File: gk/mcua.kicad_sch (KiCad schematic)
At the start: 16 parts, among them SW1 SW_Push, SW2 SW_Push, U4 STM32H747BITx, Y1 16MHz

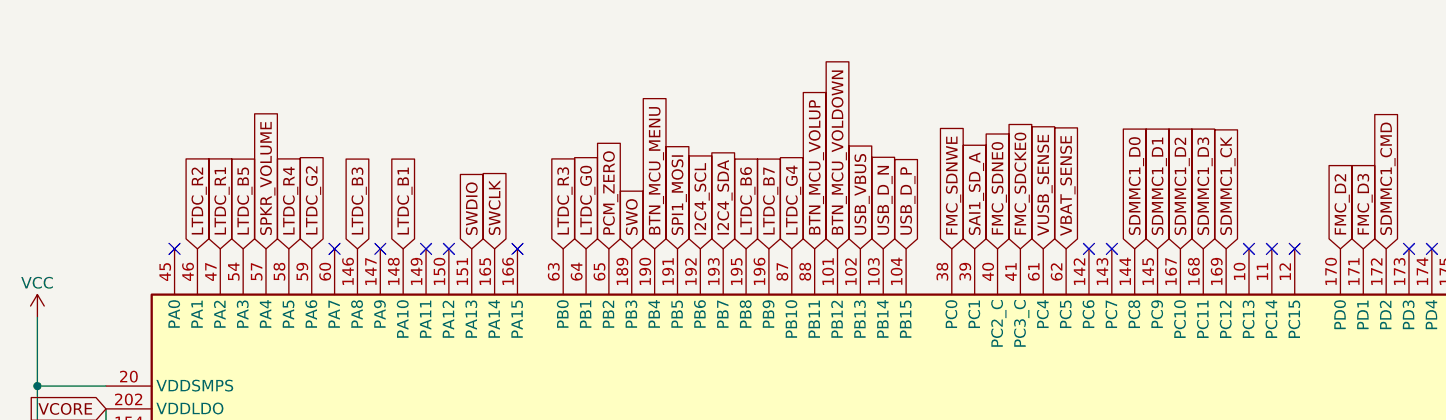
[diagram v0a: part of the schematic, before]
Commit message: Update pcb
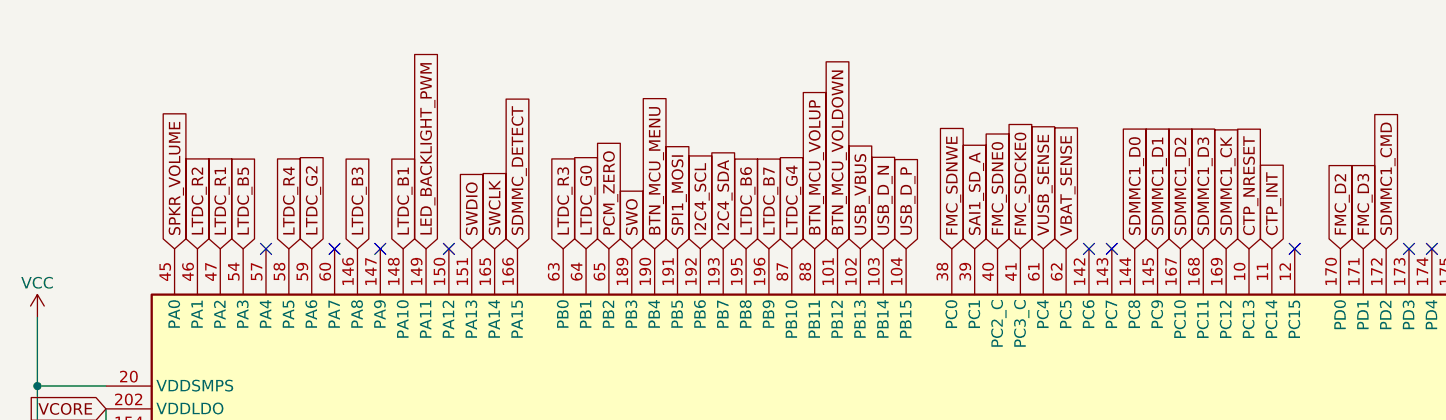
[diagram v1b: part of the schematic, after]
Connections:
- net SPKR_VOLUME: now also U4.45 (PA0); no longer U4.57 (PA4)
- net CTP_NRESET: now reaches U4.10 (PC13)
- net CTP_INT: now reaches U4.11 (PC14)
- net LED_BACKLIGHT_PWM: now reaches U4.149 (PA11)
- net SDMMC_DETECT: now reaches U4.166 (PA15)
- no-connect marks 26 -> 22
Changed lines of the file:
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@@
   (no_connect (at 68.58 146.05))
   (no_connect (at 71.12 146.05))
-  (no_connect (at 73.66 49.53))
-  (no_connect (at 35.56 49.53))
   (no_connect (at 99.06 146.05))
   (no_connect (at 139.7 49.53))
+  (no_connect (at 45.72 49.53))
   (no_connect (at 175.26 49.53))
   (no_connect (at 172.72 49.53))
@@
   (no_connect (at 165.1 146.05))
   (no_connect (at 63.5 146.05))
-  (no_connect (at 154.94 49.53))
   (no_connect (at 66.04 146.05))
-  (no_connect (at 63.5 49.53))
-  (no_connect (at 157.48 49.53))
   (no_connect (at 50.8 146.05))
   (no_connect (at 160.02 49.53))
@@
     )
   )
+  (global_label "CTP_INT" (shape input) (at 157.48 49.53 90) (fields_autoplaced)
+    (effects (font (size 1.27 1.27)) (justify left))
+    (property "Intersheetrefs" "${INTERSHEET_REFS}" (at 157.48 39.2461 90)
+      (effects (font (size 1.27 1.27)) (justify left) hide)
+    )
+  )
   (global_label "WIFI_CHIP_EN" (shape input) (at 195.58 49.53 90) (fields_autoplaced)
     (effects (font (size 1.27 1.27)) (justify left))
@@
     )
   )
+  (global_label "LED_BACKLIGHT_PWM" (shape input) (at 63.5 49.53 90) (fields_autoplaced)
+    (effects (font (size 1.27 1.27)) (justify left))
+    (property "Intersheetrefs" "${INTERSHEET_REFS}" (at 63.5 26.9695 90)
+      (effects (font (size 1.27 1.27)) (justify left) hide)
+    )
+  )
   (global_label "PCM_FMT" (shape input) (at 88.9 146.05 270) (fields_autoplaced)
     (effects (font (size 1.27 1.27)) (justify right))
@@
     )
   )
-  (global_label "SPKR_VOLUME" (shape input) (at 45.72 49.53 90) (fields_autoplaced)
-    (effects (font (size 1.27 1.27)) (justify left))
-    (property "Intersheetrefs" "${INTERSHEET_REFS}" (at 45.72 33.259 90)
-      (effects (font (size 1.27 1.27)) (justify left) hide)
-    )
-  )
   (global_label "FMC_BA1" (shape input) (at 170.18 146.05 270) (fields_autoplaced)
     (effects (font (size 1.27 1.27)) (justify right))
@@
     )
   )
+  (global_label "CTP_NRESET" (shape input) (at 154.94 49.53 90) (fields_autoplaced)
+    (effects (font (size 1.27 1.27)) (justify left))
+    (property "Intersheetrefs" "${INTERSHEET_REFS}" (at 154.94 35.0734 90)
+      (effects (font (size 1.27 1.27)) (justify left) hide)
+    )
+  )
   (global_label "LTDC_HYSNC" (shape input) (at 104.14 146.05 270) (fields_autoplaced)
     (effects (font (size 1.27 1.27)) (justify right))
@@
       (effects (font (size 1.27 1.27)) (justify left) hide)
     )
+  )
+  (global_label "SPKR_VOLUME" (shape input) (at 35.56 49.53 90) (fields_autoplaced)
+    (effects (font (size 1.27 1.27)) (justify left))
+    (property "Intersheetrefs" "${INTERSHEET_REFS}" (at 35.56 33.259 90)
+      (effects (font (size 1.27 1.27)) (justify left) hide)
+    )
+  )
+  (global_label "SDMMC_DETECT" (shape input) (at 73.66 49.53 90) (fields_autoplaced)
+    (effects (font (size 1.27 1.27)) (justify left))
+    (property "Intersheetrefs" "${INTERSHEET_REFS}" (at 73.66 32.2311 90)
+      (effects (font (size 1.27 1.27)) (justify left) hide)
+    )

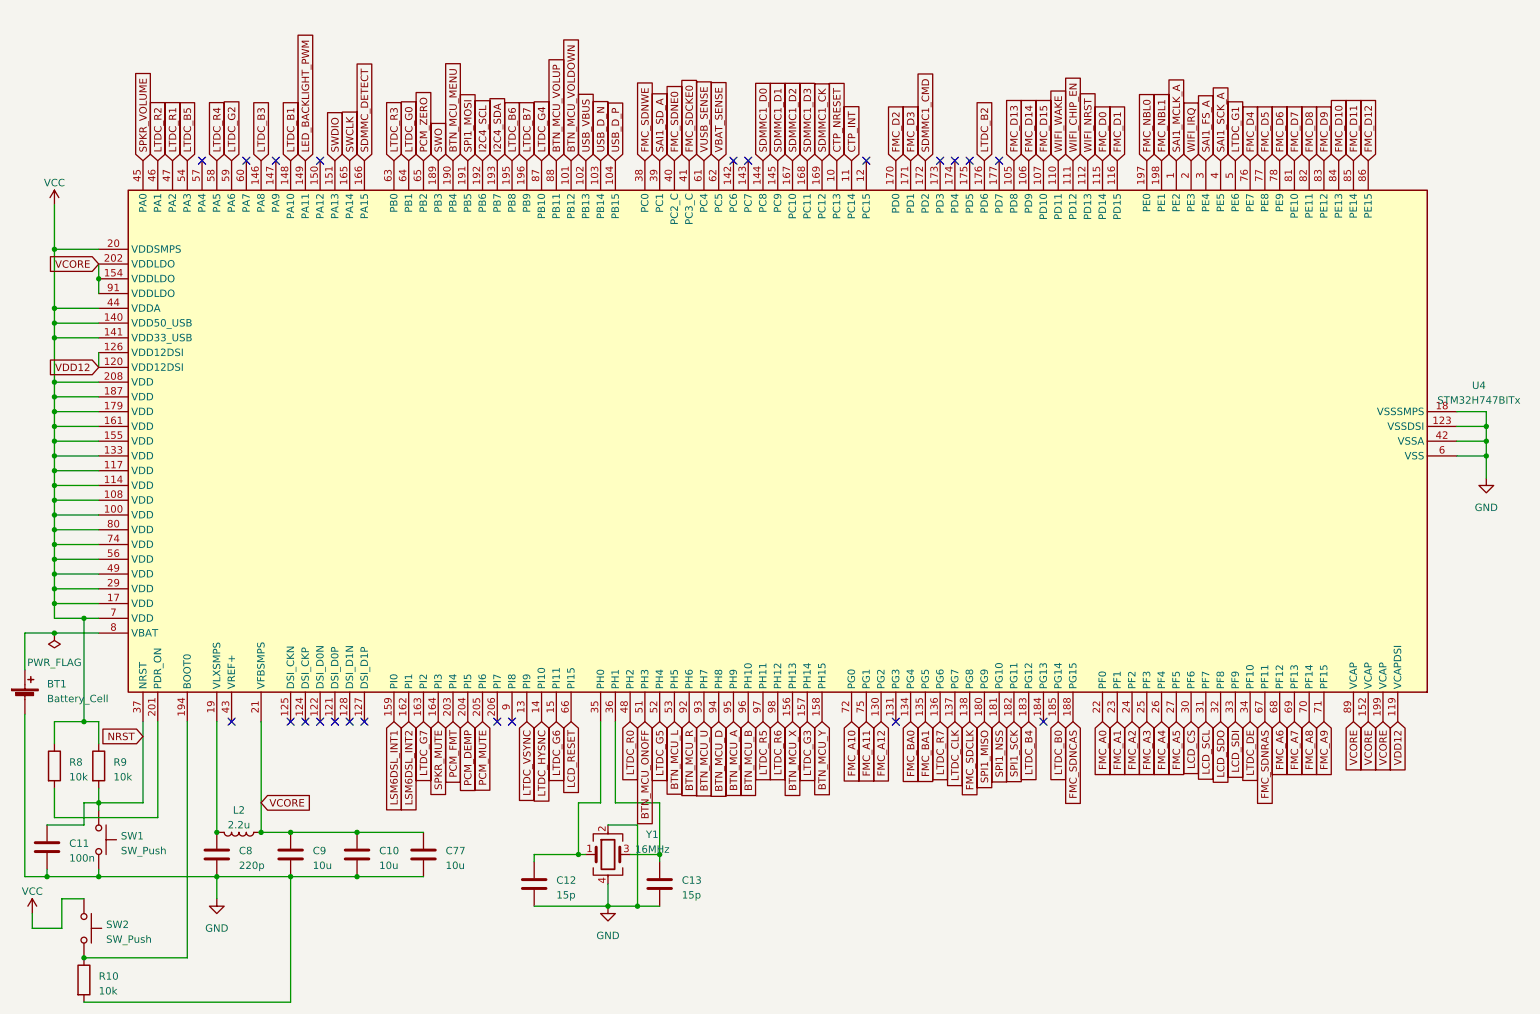
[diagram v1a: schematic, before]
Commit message: Update pcb
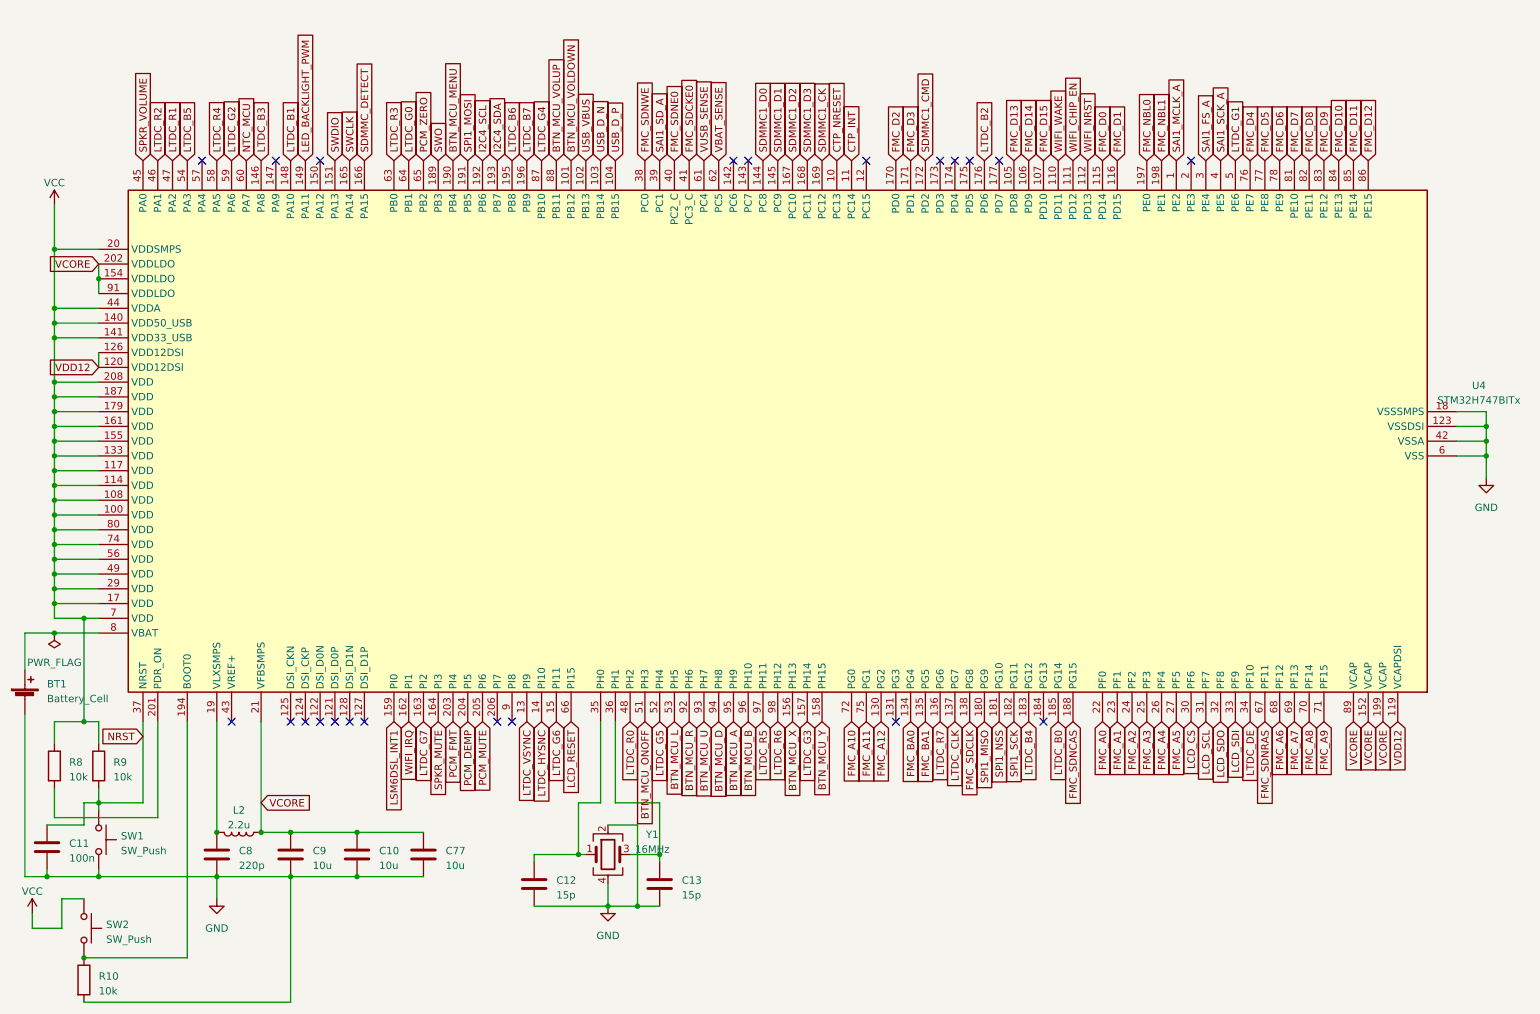
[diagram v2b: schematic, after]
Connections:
- net LSM6DSL_INT2 is gone; now on net WIFI_IRQ: U4.162 (PI1)
- net WIFI_IRQ: no longer U4.2 (PE3)
- net NTC_MCU: now reaches U4.60 (PA7)
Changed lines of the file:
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@@
   (no_connect (at 99.06 146.05))
   (no_connect (at 139.7 49.53))
+  (no_connect (at 215.9 49.53))
   (no_connect (at 45.72 49.53))
   (no_connect (at 175.26 49.53))
@@
   (no_connect (at 60.96 146.05))
   (no_connect (at 182.88 49.53))
-  (no_connect (at 53.34 49.53))
   (no_connect (at 137.16 49.53))
   (no_connect (at 177.8 49.53))
@@
     )
   )
-  (global_label "WIFI_IRQ" (shape input) (at 215.9 49.53 90) (fields_autoplaced)
-    (effects (font (size 1.27 1.27)) (justify left))
-    (property "Intersheetrefs" "${INTERSHEET_REFS}" (at 215.9 38.7017 90)
-      (effects (font (size 1.27 1.27)) (justify left) hide)
-    )
-  )
   (global_label "BTN_MCU_R" (shape input) (at 129.54 146.05 270) (fields_autoplaced)
     (effects (font (size 1.27 1.27)) (justify right))
@@
     )
   )
-  (global_label "LSM6DSL_INT2" (shape input) (at 81.28 146.05 270) (fields_autoplaced)
-    (effects (font (size 1.27 1.27)) (justify right))
-    (property "Intersheetrefs" "${INTERSHEET_REFS}" (at 81.28 162.4419 90)
-      (effects (font (size 1.27 1.27)) (justify right) hide)
-    )
-  )
   (global_label "VDD12" (shape input) (at 27.94 85.09 180) (fields_autoplaced)
     (effects (font (size 1.27 1.27)) (justify right))
@@
     )
   )
+  (global_label "NTC_MCU" (shape input) (at 53.34 49.53 90) (fields_autoplaced)
+    (effects (font (size 1.27 1.27)) (justify left))
+    (property "Intersheetrefs" "${INTERSHEET_REFS}" (at 53.34 38.0366 90)
+      (effects (font (size 1.27 1.27)) (justify left) hide)
+    )
+  )
   (global_label "FMC_A12" (shape input) (at 162.56 146.05 270) (fields_autoplaced)
     (effects (font (size 1.27 1.27)) (justify right))
@@
     )
   )
+  (global_label "WIFI_IRQ" (shape input) (at 81.28 146.05 270) (fields_autoplaced)
+    (effects (font (size 1.27 1.27)) (justify right))
+    (property "Intersheetrefs" "${INTERSHEET_REFS}" (at 81.28 156.8783 90)
+      (effects (font (size 1.27 1.27)) (justify right) hide)
+    )
+  )
